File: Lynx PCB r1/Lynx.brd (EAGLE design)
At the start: 150 x 50.1 mm, 78 parts, among them IC1 MCP1703DB, Q1 8MHz, X1 BU-SMA-V, X2 332-02, X3 332-02

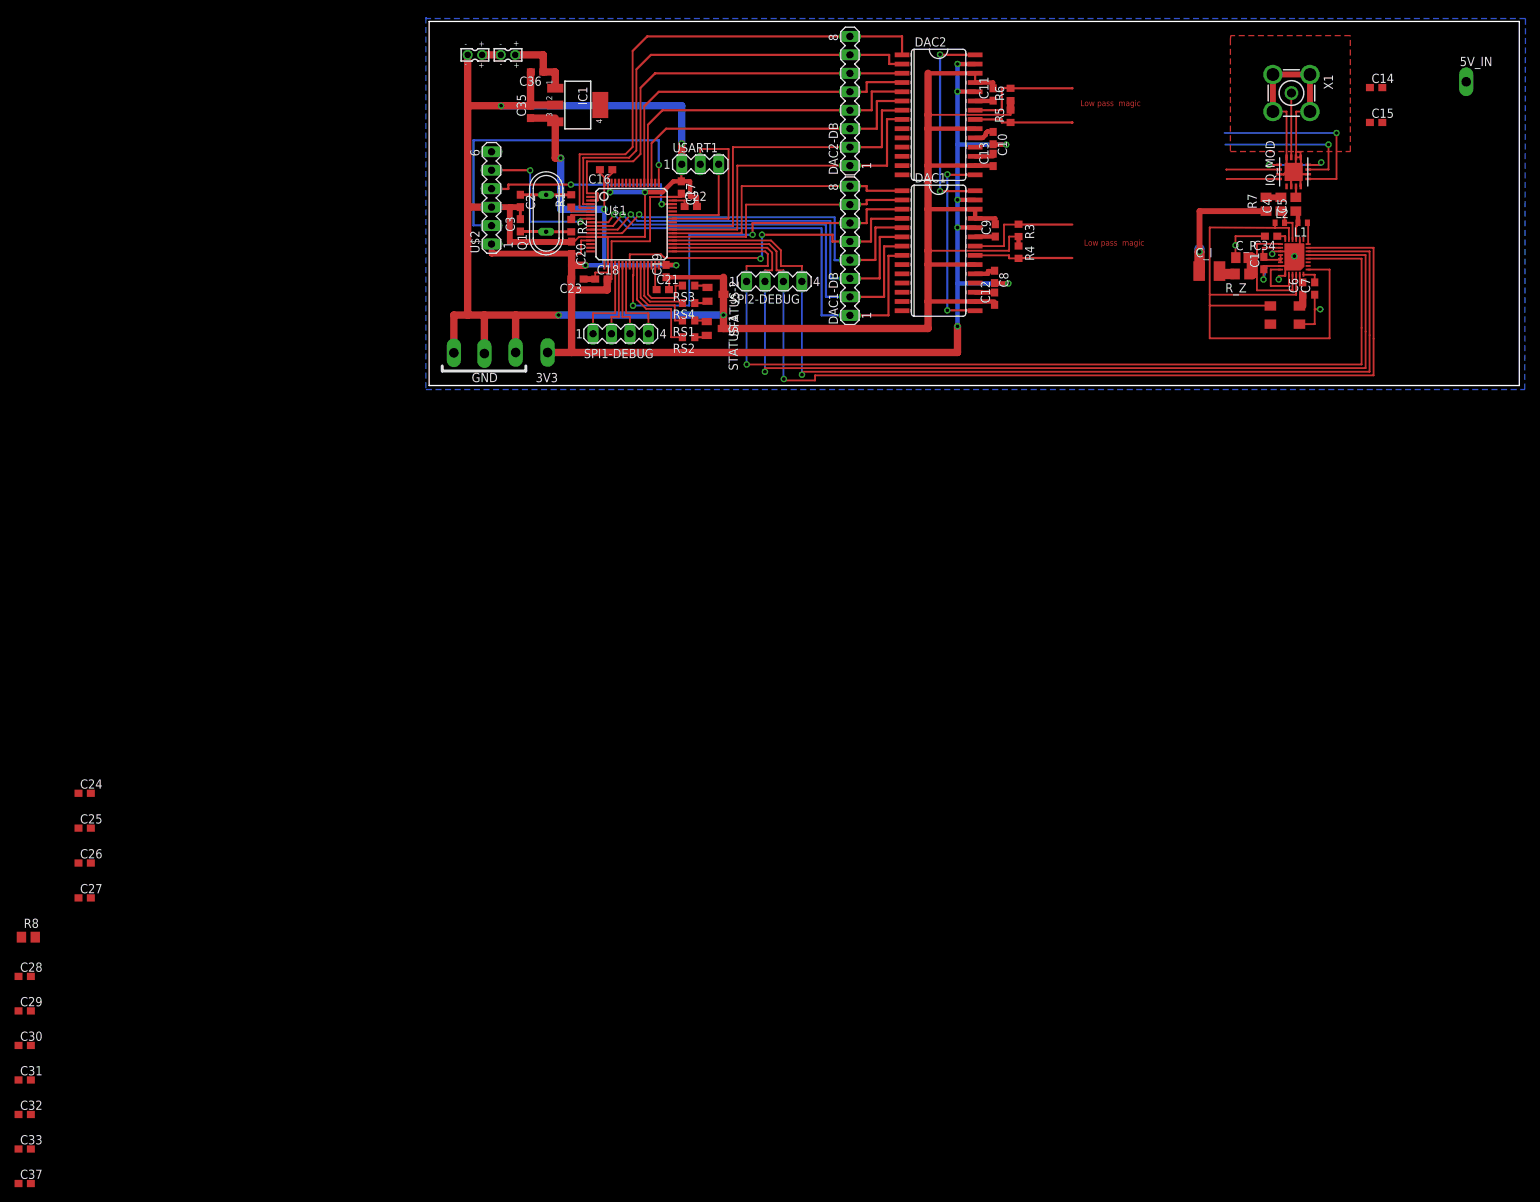
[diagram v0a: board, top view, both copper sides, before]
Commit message: rf routing
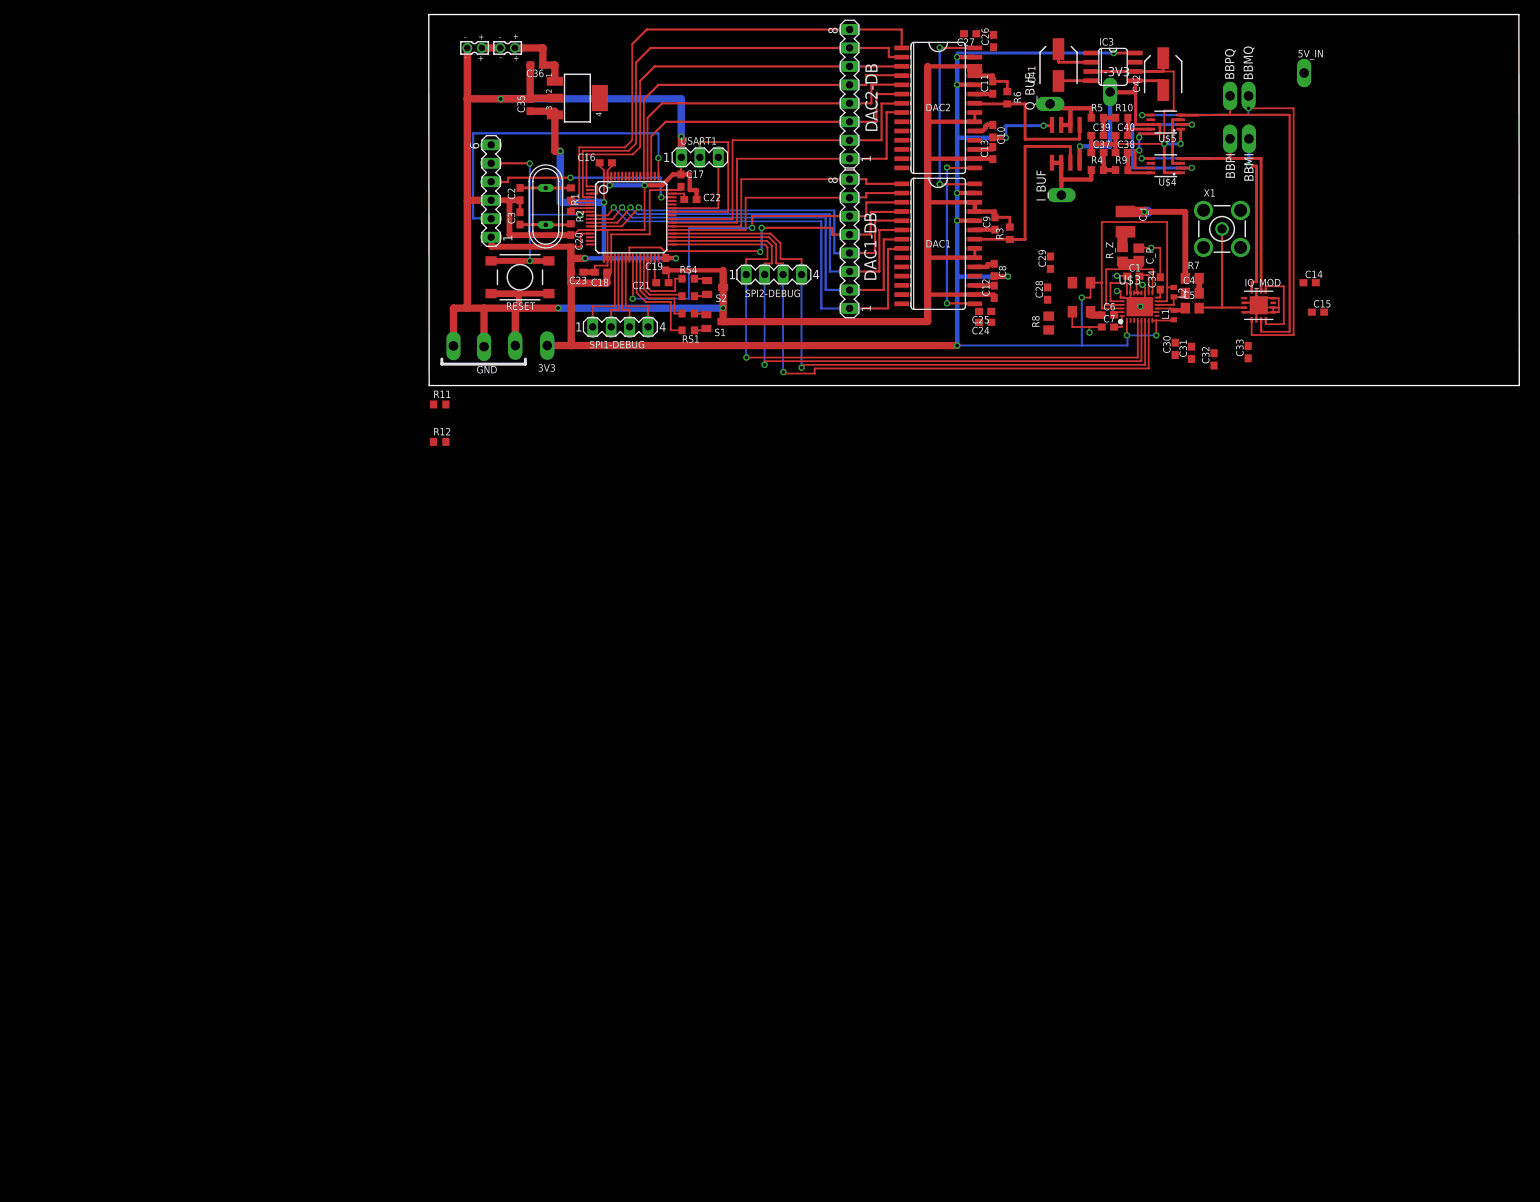
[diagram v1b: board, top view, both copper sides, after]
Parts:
- removed STATUS-1, STATUS-2: BI-LED-CC, Lynx components:SOT-23
- added -3V3, BBMI, BBMQ, BBPI, BBPQ, I_BUF, Q_BUF: PTR1PAD1-13Y, testpad:P1-13Y
- added C38, C39, C40: 150pF, rcl:C0603
- added C41, C42: 10uF, rcl:SANYO-OSCON_SMD_B6
- added IC2: (no value), linear:SO08
- added IC3: ICL7660, maxim:SO08
- added R10, R11, R12, R9: 1500, resistor:R0603
- added RESET: DTSM-6, switch-tact:DTSM-6
- added S1, S2: BI-LED-CC, Lynx components:SOT-23
- added U$4, U$5: AD8476, Lynx components:MSOP8
- C37: value 0.1uF -> 150pF
- R3, R6: value 50 -> 100
- R4, R5: value 50 -> 1500
- moved C37 204.7 mm to (92.0, 32.0)
- moved C33 200.9 mm to (112.7, 4.60), turned to 90 degrees
- moved C32 193.8 mm to (108.0, 3.60), turned to 90 degrees
- moved C31 189.2 mm to (104.9, 4.50), turned to 90 degrees
- moved C30 185.1 mm to (102.7, 5.05), turned to 90 degrees
- moved C29 174.7 mm to (85.5, 16.9), turned to 90 degrees
- moved C27 170.2 mm to (74.5, 48.4), turned to 180 degrees
- moved C28 169.2 mm to (85.1, 12.7), turned to 90 degrees
- moved C26 168.6 mm to (77.7, 47.4), turned to 90 degrees
- moved R8 163.9 mm to (85.2, 8.60), turned to 90 degrees
- moved C25 142.9 mm to (76.5, 10.2), turned to 180 degrees
- moved C24 139.8 mm to (76.5, 8.70), turned to 180 degrees
- moved C7 28.9 mm to (93.4, 8.05), turned to 0 degrees
- moved C14 28.4 mm to (121.2, 14.2)
- moved 10MHZ 28.1 mm to (89.8, 12.2), turned to 270 degrees
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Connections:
- removed net MOD-RF: IQ_MOD.11, X1.1
- new net +0.54V: R11.1, R12.2, U$4.3, U$5.3
- new net -3V3: -3V3.TP, C42.-, IC2.4, IC3.5, U$4.7, U$5.7
- new net GND1: IC2.1, IC2.2, I_BUF.TP, R4.1
- new net GND2: IC2.6, IC2.7, Q_BUF.TP, R5.1
- new net N$14: DAC1.22, IC2.3, R3.1
- new net N$29: DAC2.22, IC2.5, R6.2
- new net N$31: C37.2, R4.2, R9.1
- new net N$32: C38.2, R9.2, U$4.8
- new net N$34: C41.-, IC3.4
- new net N$35: C39.2, R10.1, R5.2
- new net N$36: C40.2, R10.2, U$5.8
- new net N$37: C41.+, IC3.2
- net +3V3: now also IC2.8, IC3.8, R11.2, U$4.2, U$5.2; no longer C37.1
- net BBMI: now also BBMI.TP, U$4.5; no longer DAC1.21, R4.2
- net BBMQ: now also BBMQ.TP, U$5.5; no longer DAC2.22, R6.2
- net BBPI: now also BBPI.TP, U$4.4; no longer DAC1.22, R3.1
- net BBPQ: now also BBPQ.TP, U$5.4; no longer DAC2.21, R5.1
- net GND: now also C37.1, C38.1, C39.1, C40.1, C42.+, DAC1.21, DAC2.21, IC3.3, IC3.6, R12.1, RESET.3, RESET.4, S1.3, S2.3, U$4.1, U$5.1; no longer C37.2, R4.1, R5.2, STATUS-1.3, STATUS-2.3
- net LO: now also X1.1
- net N$16: now also S1.1; no longer STATUS-1.1
- net N$17: now also S1.2; no longer STATUS-1.2
- net N$18: now also S2.1; no longer STATUS-2.1
- net N$19: now also S2.2; no longer STATUS-2.2
- net NRST: now also RESET.1, RESET.2
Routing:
- net +3V3: track 320.1 -> 383.9 mm, vias 11 -> 18
- net SPI2-MISO: track 141.9 -> 91.0 mm
- net SPI2-MOSI: track 139.0 -> 89.2 mm
- net SPI2-SCK: track 138.0 -> 89.3 mm
- net SPI2-CS: track 137.9 -> 90.4 mm
- net -3V3: track 0.00 -> 43.9 mm, vias 0 -> 3
- net N$14: track 0.00 -> 28.2 mm
- net BBMQ: track 42.2 -> 63.8 mm, vias 1 -> 2
- net N$29: track 0.00 -> 21.3 mm
- net BBPQ: track 34.3 -> 53.1 mm, vias 1 -> 0
- net BBMI: track 21.1 -> 38.8 mm, vias 0 -> 2
- net LO: track 2.00 -> 17.4 mm
- net NRST: track 21.1 -> 35.4 mm, vias 2 -> 3
- net GND: track 476.0 -> 490.2 mm, vias 12 -> 14
- net GND2: track 0.00 -> 11.3 mm
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- removed copper zone on layer 16, net GND
- removed copper zone on layer 1, net N$14
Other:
- board size 150 x 50.1 mm -> 150.1 x 51 mm
- board text removed: "Low pass magic"
